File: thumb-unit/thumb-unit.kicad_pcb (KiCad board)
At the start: 2 copper layers, 82.5 x 79 mm, 0 parts

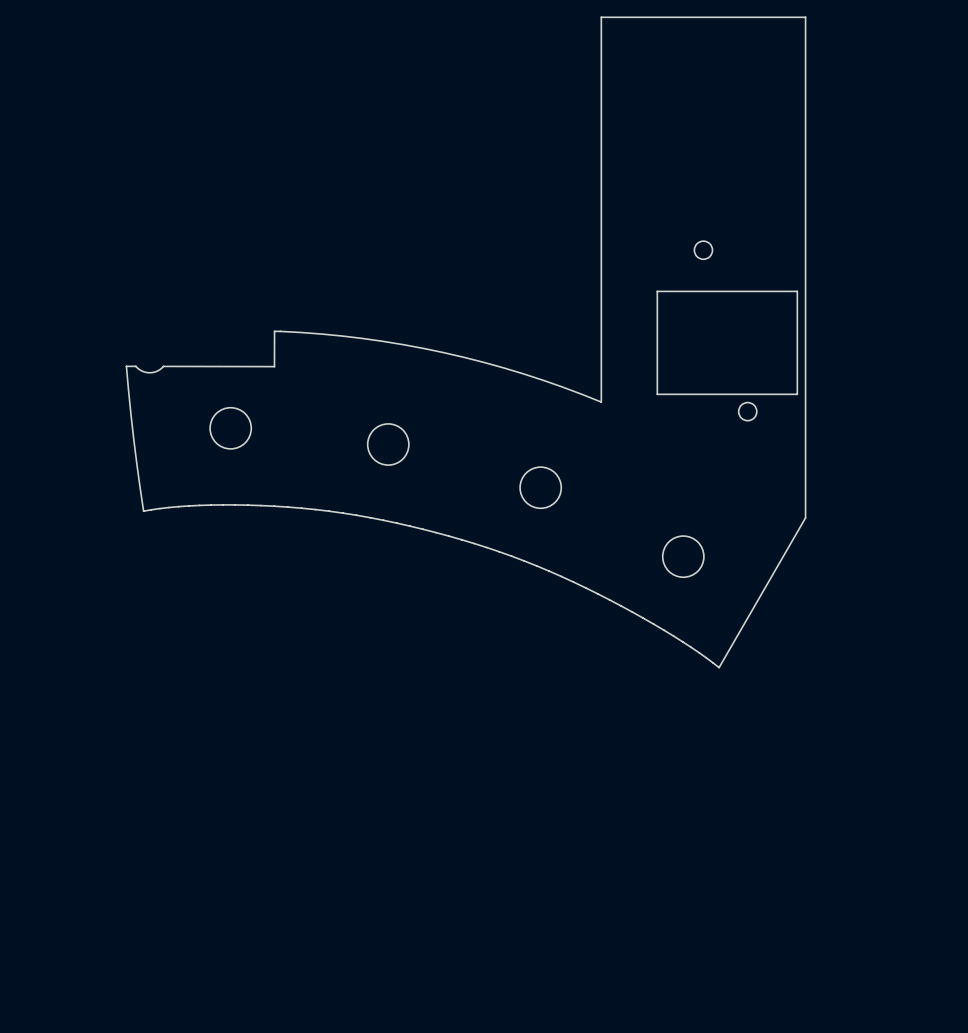
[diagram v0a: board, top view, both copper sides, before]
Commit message: feat: 親指ユニット・一旦完成
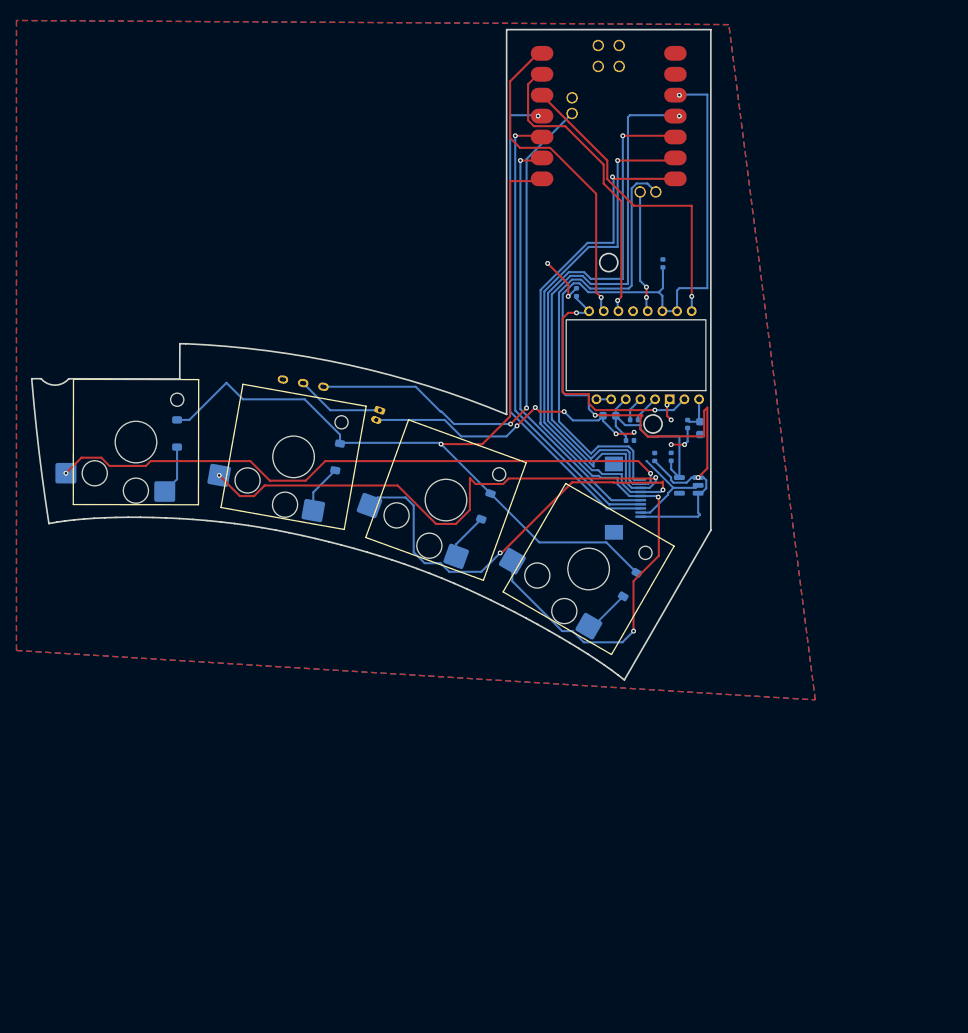
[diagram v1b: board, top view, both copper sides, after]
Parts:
- added BT1: Battery, Connector_Molex:Molex_PicoBlade_53048-0210_1x02_P1.25mm_Horizontal, B.Cu at (134.6, 106.3)
- added C1: 1uF, Capacitor_SMD:C_0402_1005Metric, B.Cu at (168.0, 112.0)
- added C10: 10uF X7R, Capacitor_SMD:C_0603_1608Metric, B.Cu at (173.5, 108.5)
- added C11: 10nF X7R, Capacitor_SMD:C_0402_1005Metric, B.Cu at (172.0, 108.0)
- added C12: 10nF, Capacitor_SMD:C_0402_1005Metric, B.Cu at (158.5, 92.0)
- added C13: 100nF X7R, Capacitor_SMD:C_0402_1005Metric, B.Cu at (165.5, 107.5)
- added C15: 100nF, Capacitor_SMD:C_0402_1005Metric, B.Cu at (169.0, 88.5)
- added C16: 100nF, Capacitor_SMD:C_0402_1005Metric, B.Cu at (165.0, 110.0)
- added C17: 3.3uF/16V, Capacitor_SMD:C_0603_1608Metric, B.Cu at (162.5, 107.0)
- added C2: 1uf, Capacitor_SMD:C_0402_1005Metric, B.Cu at (170.0, 112.0)
- added D1: D, Diode_SMD:D_SOD-123, B.Cu at (165.0, 127.5)
- added D2: D, Diode_SMD:D_SOD-123, B.Cu at (147.5, 118.0)
- added D3: D, Diode_SMD:D_SOD-123, B.Cu at (129.5, 112.0)
- added D4: D, Diode_SMD:D_SOD-123, B.Cu at (110.0, 109.2)
- added J1: Conn_01x10, Connector_FFC-FPC:Hirose_FH12-10S-0.5SH_1x10-1MP_P0.50mm_Horizontal, B.Cu at (164.4, 117.0)
- added SW1: SW_SPDT, custom:TGSW_MSK-12D19, B.Cu at (125.5, 102.0)
- added SW2: SW_Push, PCM_Switch_Keyboard_Hotswap_Kailh:SW_Hotswap_Kailh_Choc_V2_1.00u, F.Cu at (160.0, 125.6)
- added SW3: SW_Push, PCM_Switch_Keyboard_Hotswap_Kailh:SW_Hotswap_Kailh_Choc_V2_1.00u, F.Cu at (142.7, 117.2)
- added SW4: SW_Push, PCM_Switch_Keyboard_Hotswap_Kailh:SW_Hotswap_Kailh_Choc_V2_1.00u, F.Cu at (124.1, 112.0)
- added SW5: SW_Push, PCM_Switch_Keyboard_Hotswap_Kailh:SW_Hotswap_Kailh_Choc_V2_1.00u, F.Cu at (105.0, 110.2)
- added U1: xiao-ble, mcu:xiao-ble-smd, F.Cu at (162.4, 70.6)
- added U2: PMW3610, sensor:PMW3610, B.Cu at (164.3, 99.6)
- added U3: TLV70218_SOT23-5, Package_TO_SOT_SMD:SOT-23-5, B.Cu at (172.1, 115.5)
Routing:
- net /COL3: track 0.00 -> 146.8 mm, vias 0 -> 3
- net /COL2: track 0.00 -> 132.9 mm, vias 0 -> 3
- net +3V3: track 0.00 -> 119.8 mm, vias 0 -> 3
- net /COL1: track 0.00 -> 112.4 mm, vias 0 -> 3
- net /ROW3: track 0.00 -> 109.8 mm, vias 0 -> 1
- net /COL0: track 0.00 -> 100.6 mm, vias 0 -> 3
- net /BAT_SW: track 0.00 -> 65.4 mm, vias 0 -> 2
- net GND: track 0.00 -> 62.0 mm, vias 0 -> 11
- net /ROW0: track 0.00 -> 60.1 mm, vias 0 -> 1
- net /COL4: track 0.00 -> 56.7 mm
- net /ROW1: track 0.00 -> 56.2 mm, vias 0 -> 1
- net /ROW2: track 0.00 -> 51.7 mm, vias 0 -> 1
- net /SDIO: track 0.00 -> 39.6 mm, vias 0 -> 1
- net /MOTION: track 0.00 -> 38.3 mm, vias 0 -> 1
- net /SCLK: track 0.00 -> 36.4 mm, vias 0 -> 1
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- added copper zone on B.Cu, net GND
- added copper zone on F.Cu, net GND
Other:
- outline, holes or cut-outs redrawn

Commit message: feat: 回路図完成
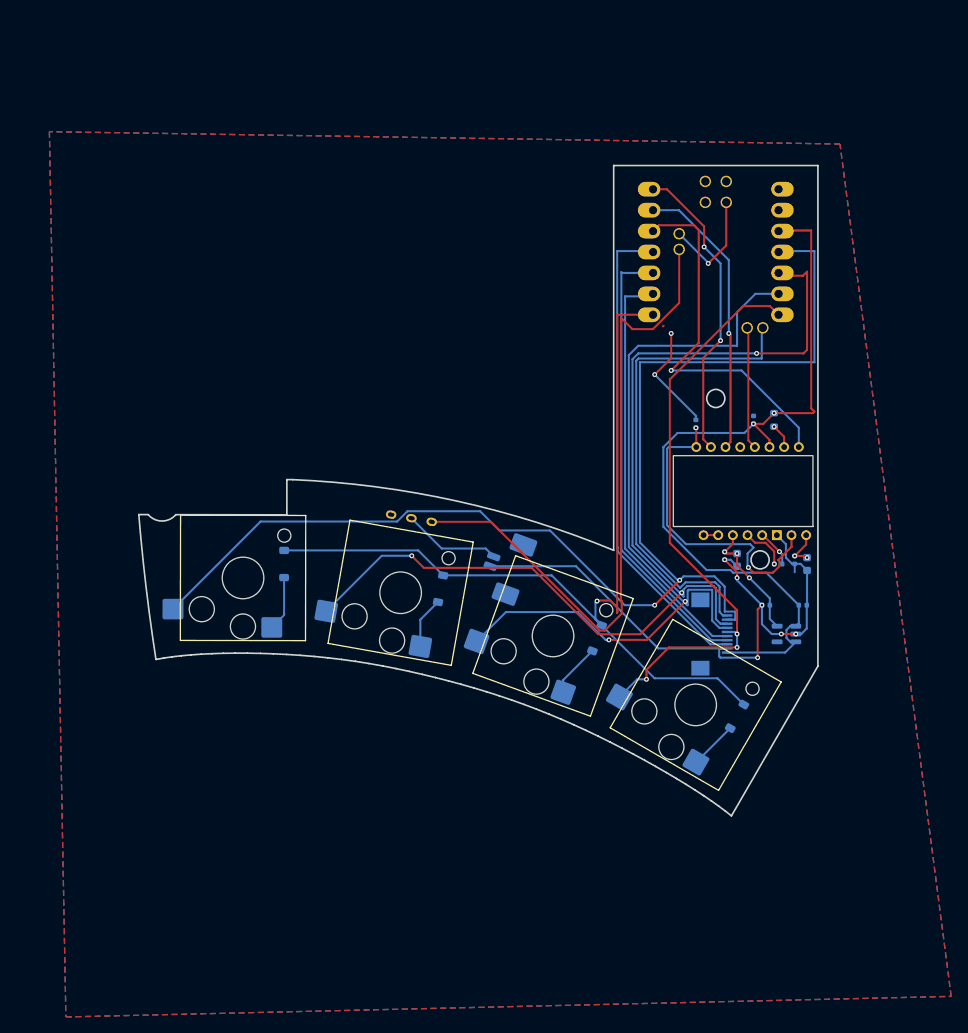
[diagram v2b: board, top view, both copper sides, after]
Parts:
- added R1: 10k, Resistor_SMD:R_0603_1608Metric, B.Cu at (182.5, 107.5)
- BT1: footprint Connector_Molex:Molex_PicoBlade_53048-0210_1x02_P1.25mm_Horizontal -> Connector_Molex:Molex_PicoBlade_53261-0271_1x02-1MP_P1.25mm_Horizontal
- U1: footprint mcu:xiao-ble-smd -> mcu:xiao-ble-tht
- moved C1 25.4 mm to (186.0, 130.0), turned to 180 degrees
- moved BT1 24.9 mm to (150.5, 125.5)
- moved C13 24.7 mm to (183.0, 125.0)
- moved C17 23.4 mm to (178.0, 124.5), turned to -90 degrees
- moved C15 22.0 mm to (180.0, 107.5)
- moved U3 21.6 mm to (184.0, 133.5)
- moved C12 21.6 mm to (173.0, 108.0)
- moved C2 21.4 mm to (181.5, 130.0), turned to 0 degrees
- moved SW1 21.0 mm to (138.6, 118.4)
- moved U1 21.0 mm to (175.4, 87.1)
- moved U2 21.0 mm to (177.3, 116.1)
- moved C10 21.0 mm to (186.5, 125.0)
- moved C11 21.0 mm to (185.0, 124.5)
- moved SW2 21.0 mm to (173.0, 142.1)
- moved SW3 21.0 mm to (155.7, 133.7)
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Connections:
- U2 pad 7: +3V3 -> Net-(U2-~{RESET})
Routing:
- net GND: track 62.0 -> 105.7 mm, vias 11 -> 9
- net /COL0: track 100.6 -> 72.0 mm
- net +3V3: track 119.8 -> 95.2 mm, vias 3 -> 2
- net /BAT_SW: track 65.4 -> 80.6 mm, vias 2 -> 0
- net /COL1: track 112.4 -> 97.9 mm, vias 3 -> 2
- net +1V8: track 22.5 -> 14.9 mm, vias 0 -> 3
- net /MOTION: track 38.3 -> 45.2 mm
- net Net-(U2-+VCSEL): track 31.9 -> 38.5 mm
- net /COL3: track 146.8 -> 152.7 mm, vias 3 -> 2
- net /COL2: track 132.9 -> 128.8 mm
- net Net-(U2-~{RESET}): track 0.00 -> 2.98 mm, vias 0 -> 1
- net /SDIO: track 39.6 -> 37.0 mm, vias 1 -> 2
- net Net-(U2-C-): track 3.02 -> 5.58 mm, vias 0 -> 1
- net /SCLK: track 36.4 -> 34.7 mm
- net /COL4: track 56.7 -> 58.3 mm
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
